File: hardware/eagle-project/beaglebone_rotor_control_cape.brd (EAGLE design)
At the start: 83.8 x 66.6 mm, 60 parts, among them IC1 TLC2264CDU, IC2 MCP4901, IC3 MAX3232ESE, IC6 TLC2264CDU, Q1 SQ2348ES-T1-GE3, Q2 SQ2348ES-T1-GE3, Q3 SQ2348ES-T1-GE3, Q4 SQ2348ES-T1-GE3, Q5 SQ2348ES-T1-GE3, Q6 SQ2348ES-T1-GE3, U1 TMH0512S, X1 BEAGLEBONE_OUTLINE, X4 DSUB9, X5 USBDEV

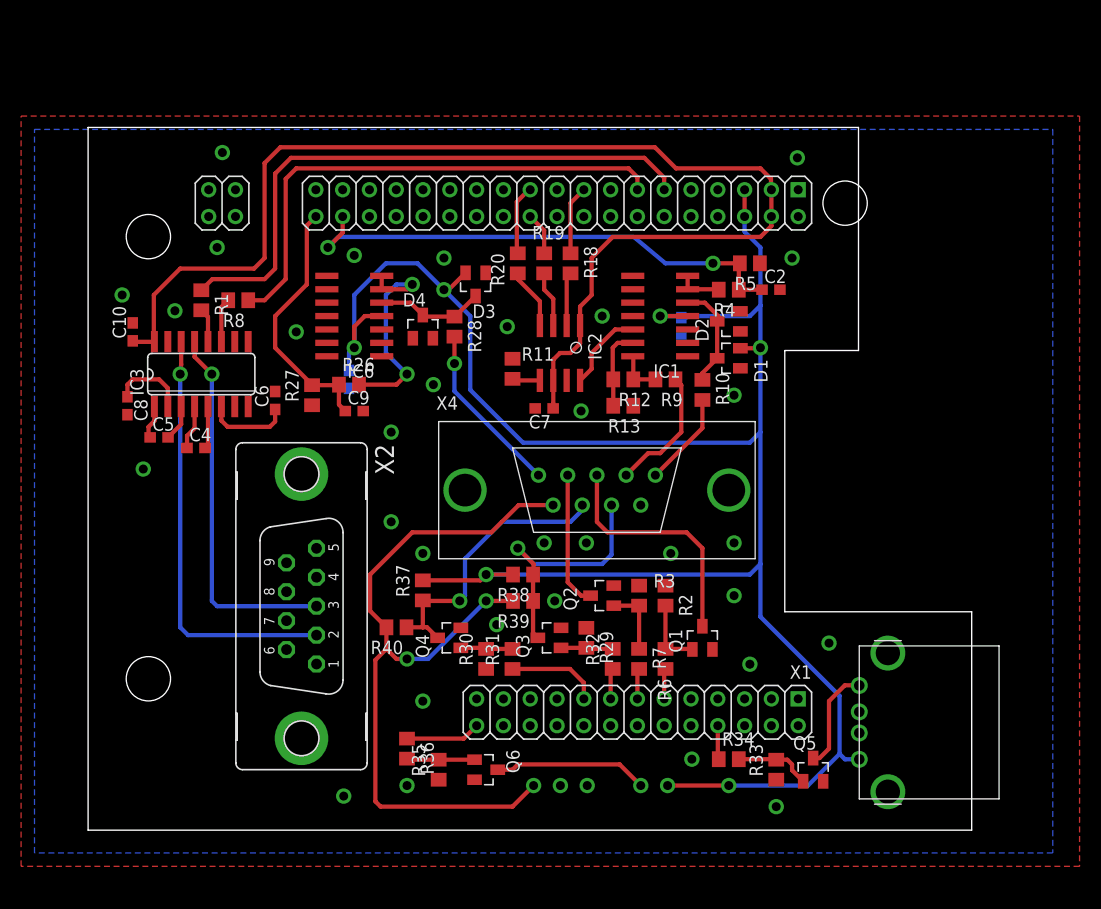
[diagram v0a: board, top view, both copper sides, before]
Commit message: Eagle layout update finalized for manufacturing
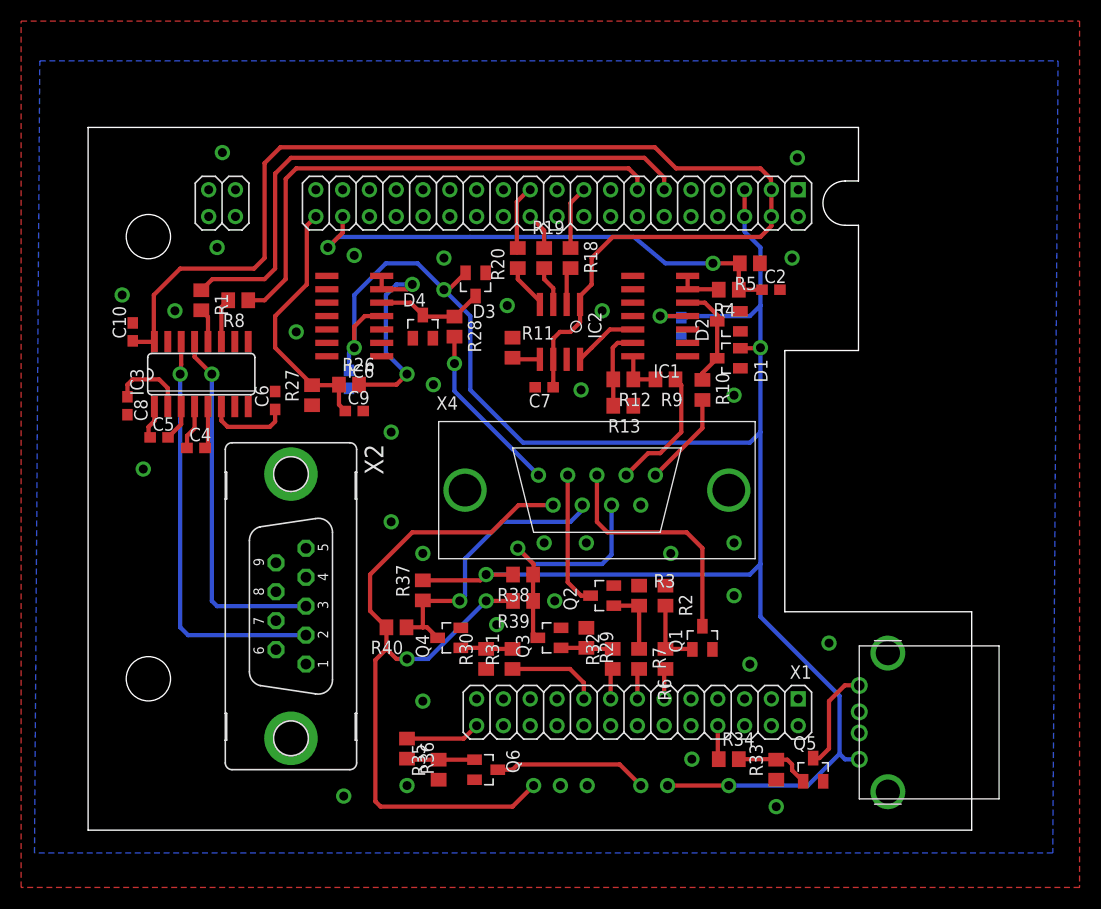
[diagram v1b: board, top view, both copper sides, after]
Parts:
- moved C7 2.00 mm to (44.5, 35.2)
- moved IC2 2.00 mm to (46.0, 40.5)
- moved R11 2.00 mm to (41.5, 39.0)
- moved X2 1.00 mm to (20.5, 14.5)
- moved R18 0.50 mm to (47.0, 47.5)
- moved R19 0.50 mm to (44.5, 47.5)
- moved R20 0.50 mm to (42.0, 47.5)
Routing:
- net +3V3: track 116.5 -> 114.5 mm
- net N$6: track 5.47 -> 3.60 mm
- net N$2: track 7.88 -> 6.17 mm
- net N$10: track 5.31 -> 3.81 mm
- net N$9: track 5.82 -> 4.32 mm
- net RS232_TX: track 40.3 -> 39.3 mm
- net RS232_RX: track 35.4 -> 34.4 mm
- net BB_SPI0_SCLK: track 4.03 -> 3.53 mm
- net BB_SPI0_CS0: track 6.55 -> 6.05 mm
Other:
- outline, holes or cut-outs redrawn
